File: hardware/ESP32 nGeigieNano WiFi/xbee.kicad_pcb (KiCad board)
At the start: 2 copper layers, 25.5 x 34.5 mm, 4 parts, among them SW1 TACT-SWITCH, U1 ESP32S

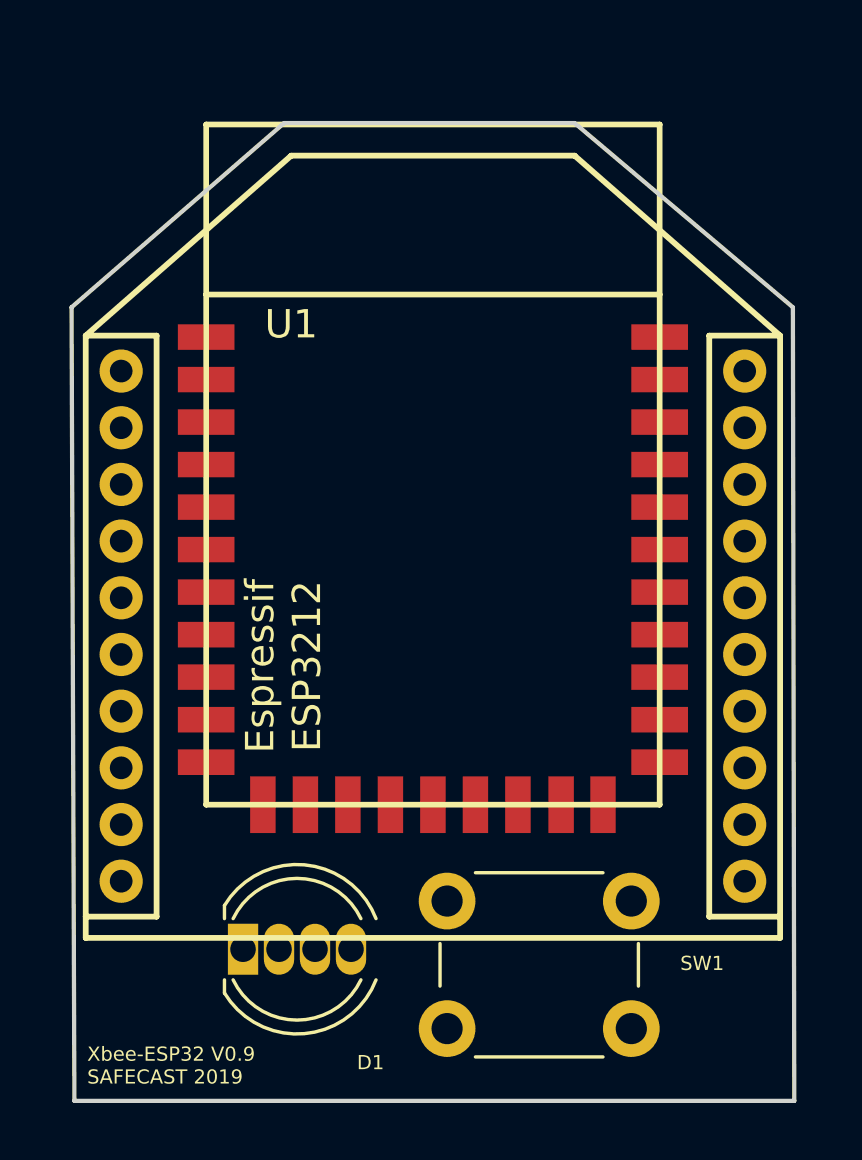
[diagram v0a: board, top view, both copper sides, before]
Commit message: add hardware designs to development
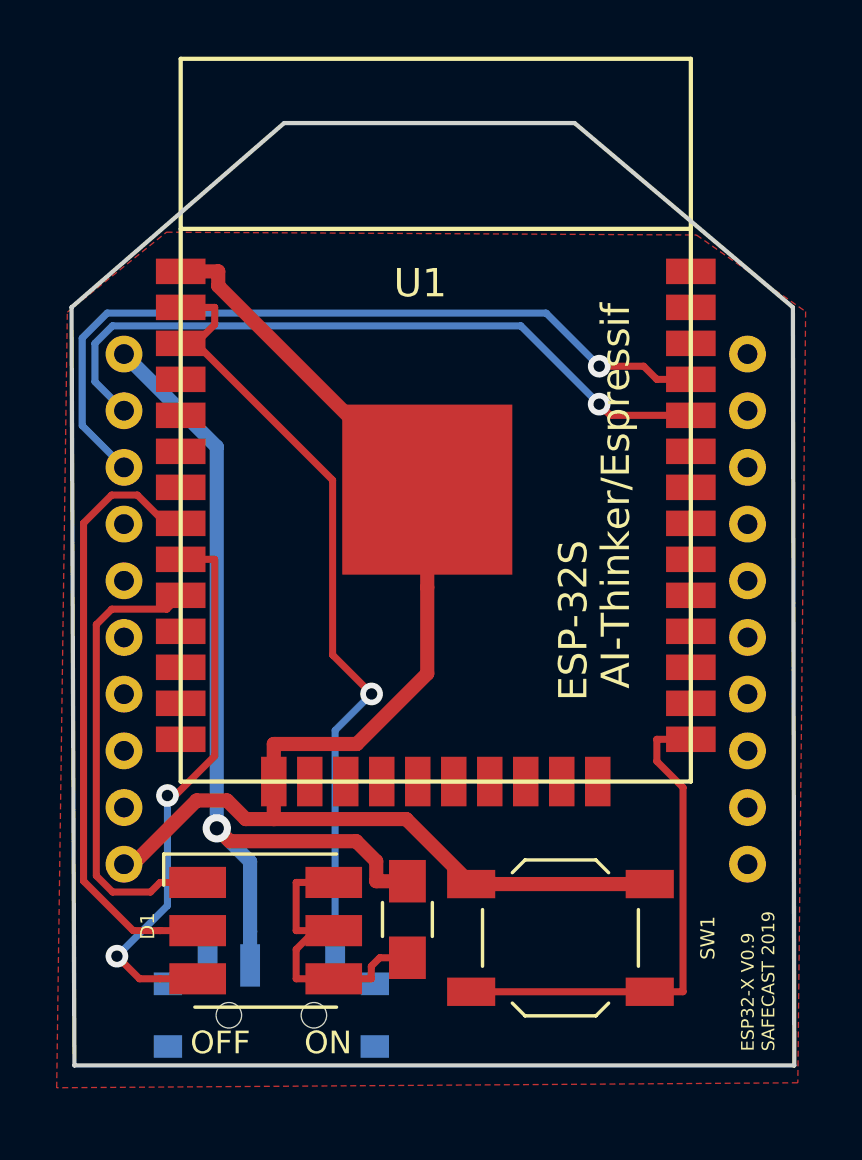
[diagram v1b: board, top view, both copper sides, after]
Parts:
- added R1: 470, Resistors_SMD:R_0805_HandSoldering, F.Cu at (147.6, 118.3)
- added SW2: SWITCH_INV, Buttons_Switches_SMD:SW_SPDT_PCM12, B.Cu at (142.8, 121.4)
- D1: footprint LEDs:LED_D5.0mm-4 -> LEDs:LED_RGB_5050-6
- SW1: footprint Buttons_Switches_THT:SW_PUSH_6mm_h4.3mm -> Buttons_Switches_SMD:SW_SPST_TL3342
- U$1: footprint XBEE-SILK -> digikey-footprints:XBEE-20_THT
- U1: footprint ESP32-footprints-Lib:ESP3212 -> ESP32-footprints-Lib:ESP-32S
- moved U$1 11.6 mm to (148.6, 107.4)
- moved SW1 4.06 mm to (153.0, 119.0)
- moved U1 2.70 mm to (148.7, 105.0)
- moved D1 1.04 mm to (142.6, 118.7)
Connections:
- SW1 pad 2: Net-(SW1-Pad2) -> GND
- U$1 pad 2: (no net) -> Net-(U$1-Pad2)
- U$1 pad 3: (no net) -> Net-(U$1-Pad3)
- U1 pad 1: Net-(U1-Pad1) -> GND
- U1 pad 10: Net-(U1-Pad10) -> Net-(D1-Pad1)
- U1 pad 11: Net-(U1-Pad11) -> (no net)
- U1 pad 12: Net-(U1-Pad12) -> (no net)
- U1 pad 13: Net-(U1-Pad13) -> (no net)
- U1 pad 14: Net-(U1-Pad14) -> (no net)
- U1 pad 15: Net-(U1-Pad15) -> GND
- U1 pad 16: Net-(U1-Pad16) -> (no net)
- U1 pad 17: Net-(U1-Pad17) -> (no net)
- U1 pad 18: Net-(U1-Pad18) -> (no net)
- U1 pad 19: Net-(U1-Pad19) -> (no net)
- U1 pad 2: Net-(U1-Pad2) -> Net-(SW2-Pad1)
- U1 pad 20: Net-(U1-Pad20) -> (no net)
- U1 pad 21: Net-(U1-Pad21) -> (no net)
- U1 pad 22: Net-(U1-Pad22) -> (no net)
- U1 pad 23: Net-(U1-Pad23) -> (no net)
- U1 pad 24: Net-(U1-Pad24) -> (no net)
- U1 pad 25: Net-(U1-Pad25) -> Net-(SW1-Pad1)
- U1 pad 26: Net-(U1-Pad26) -> (no net)
- U1 pad 27: Net-(U1-Pad27) -> (no net)
- U1 pad 28: Net-(U1-Pad28) -> (no net)
- U1 pad 29: Net-(U1-Pad29) -> (no net)
- U1 pad 3: Net-(U1-Pad3) -> Net-(SW2-Pad1)
- U1 pad 30: Net-(U1-Pad30) -> (no net)
- U1 pad 31: Net-(U1-Pad31) -> (no net)
- U1 pad 4: Net-(U1-Pad4) -> (no net)
- U1 pad 5: Net-(U1-Pad5) -> (no net)
- U1 pad 6: Net-(U1-Pad6) -> (no net)
- U1 pad 7: Net-(U1-Pad7) -> (no net)
- U1 pad 8: Net-(U1-Pad8) -> Net-(D1-Pad2)
- U1 pad 9: Net-(U1-Pad9) -> Net-(D1-Pad3)
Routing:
- net GND: track 0.00 -> 48.6 mm
- net VDD: track 0.00 -> 31.3 mm, vias 0 -> 1
- net Net-(SW2-Pad1): track 0.00 -> 28.3 mm, vias 0 -> 1
- net Net-(U$1-Pad3): track 0.00 -> 28.0 mm, vias 0 -> 1
- net Net-(U$1-Pad2): track 0.00 -> 25.4 mm, vias 0 -> 1
- net Net-(D1-Pad2): track 0.00 -> 21.6 mm
- net Net-(D1-Pad3): track 0.00 -> 20.0 mm, vias 0 -> 2
- net Net-(SW1-Pad1): track 0.00 -> 18.0 mm
- net Net-(D1-Pad1): track 0.00 -> 16.2 mm
- net Net-(D1-Pad4): track 0.00 -> 10.8 mm
- added copper zone on F.Cu, net GND
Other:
- board size 25.5 x 34.5 mm -> 25.5 x 33.2 mm
- net class Power added: clearance 0.2, trace_width 0.5, via_dia 1, via_drill 0.5
- board text added: "ESP32-X V0.9 SAFECAST 2019"
- board text added: "OFF"
- board text added: "ON"
- board text removed: "Xbee-ESP32 V0.9 SAFECAST 2019"
